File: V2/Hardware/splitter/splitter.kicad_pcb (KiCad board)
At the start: 2 copper layers, 21 parts, among them J0 Rpi_40Pin_F, J1 Control_seg:1, J2 Control_seg:2, J3 Control_seg:3, J4 Molex_PSU_F, J5 Siren, J6 USB_A_F, K0 RELRAS0515, Q1 BD139-16

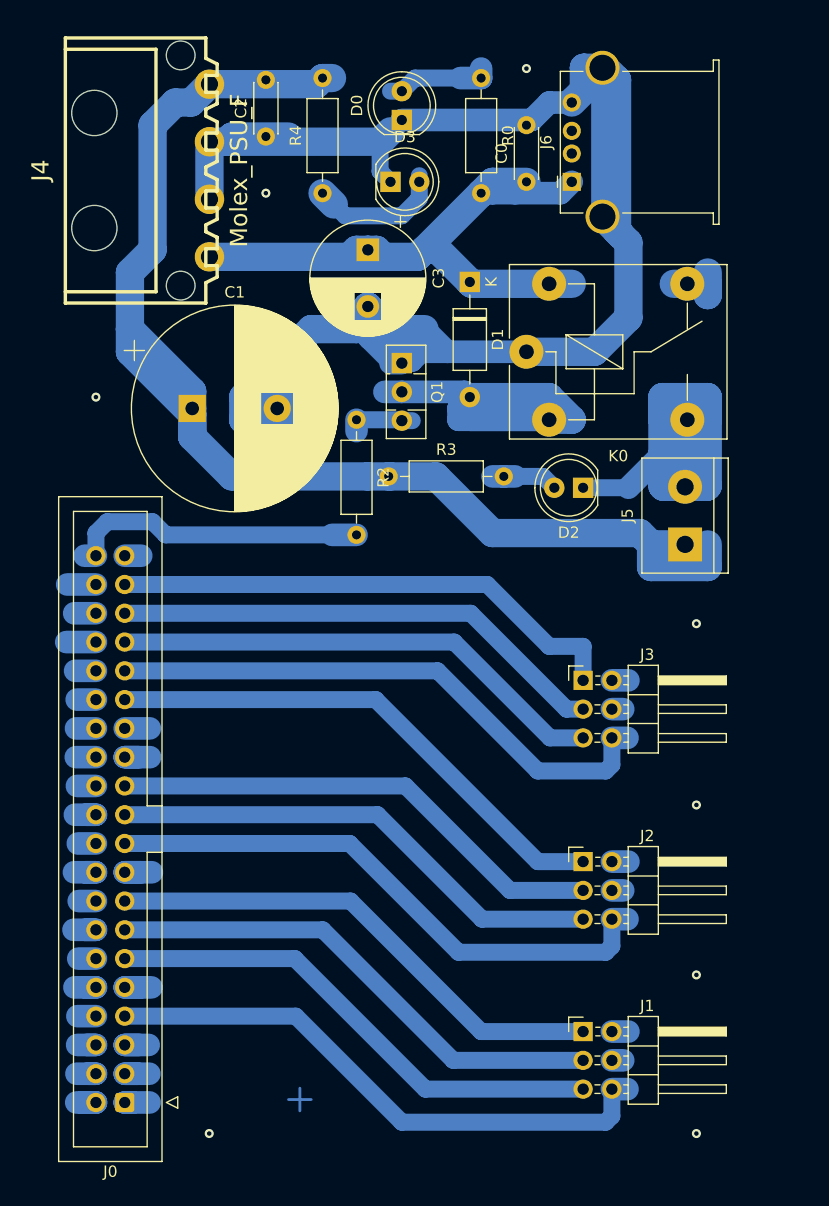
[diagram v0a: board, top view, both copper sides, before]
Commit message: Update splitter
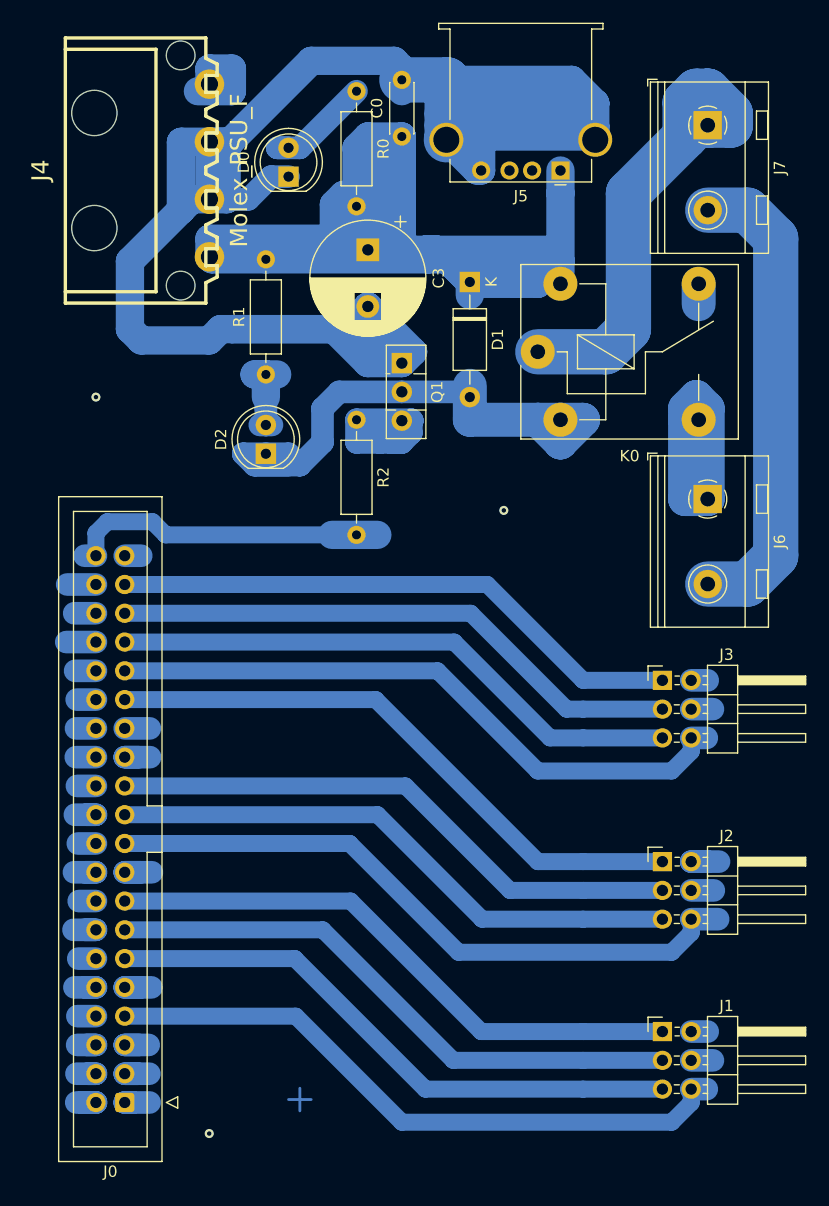
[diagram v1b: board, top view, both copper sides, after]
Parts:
- removed C1: 4700uF 25V LOW ESR, Capacitor_THT:CP_Radial_D18.0mm_P7.50mm
- removed C2: 220nF, Capacitor_THT:C_Disc_D4.3mm_W1.9mm_P5.00mm
- removed D3: LED_2V_20mA, LED_THT:LED_D5.0mm
- removed the J5 at (174.0, 83.0)
- removed R3, R4: 33k, Resistor_THT:R_Axial_DIN0207_L6.3mm_D2.5mm_P10.16mm_Horizontal
- added J6: Siren, TerminalBlock_RND:TerminalBlock_RND_205-00067_1x02_P7.50mm_Horizontal, F.Cu at (176.0, 79.0)
- added J7: Siren, TerminalBlock_RND:TerminalBlock_RND_205-00067_1x02_P7.50mm_Horizontal, F.Cu at (176.0, 46.0)
- added R1: 33k, Resistor_THT:R_Axial_DIN0207_L6.3mm_D2.5mm_P10.16mm_Horizontal, F.Cu at (137.0, 68.0)
- moved D2 28.2 mm to (137.0, 75.0), turned to 90 degrees
- moved C0 11.7 mm to (149.0, 47.0)
- moved D0 11.2 mm to (139.0, 50.5)
- moved R0 11.1 mm to (145.0, 43.0)
- moved J1 7.00 mm to (172.0, 126.0)
- moved J2 7.00 mm to (172.0, 111.0)
- moved J3 7.00 mm to (172.0, 95.0)
- moved J5 1.41 mm to (163.0, 50.0), turned to 180 degrees
- moved K0 1.00 mm to (161.0, 66.0)
- renumbered J6 to J5
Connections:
- D2 pad 1: Net-(D2-Pad1) -> Net-(D1-Pad2)
- K0 pad 11: Earth -> Net-(J7-Pad1)
- K0 pad 14: Net-(D2-Pad1) -> /230V-L
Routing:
- net /5V+: track 57.8 -> 178.5 mm
- net /12V+: track 116.5 -> 8.35 mm
- net Net-(D2-Pad1): track 47.1 -> 0.00 mm
- net Net-(J7-Pad1): track 0.00 -> 44.6 mm
- net /230V-N: track 0.00 -> 42.1 mm
- net Earth: track 190.1 -> 220.0 mm
- net Net-(D1-Pad2): track 40.0 -> 64.1 mm
- net /230V-L: track 0.00 -> 24.1 mm
- net Net-(Q1-Pad3): track 5.95 -> 22.8 mm
- net Net-(D3-Pad2): track 12.0 -> 0.00 mm
- net /seg:2_bit:a_gpio:10: track 51.0 -> 58.3 mm
- net /seg:3_bit:c_gpio:19: track 44.0 -> 51.0 mm
- net /seg:3_bit:b_gpio:13: track 44.0 -> 51.0 mm
- net /seg:2_bit:d_gpio:05: track 46.4 -> 53.4 mm
- net /seg:2_bit:c_gpio:11: track 44.3 -> 51.3 mm
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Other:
- board text added: "67mm"
- board text removed: "61mm"
